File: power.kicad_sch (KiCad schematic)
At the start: 1 part, among them U40 RP2040

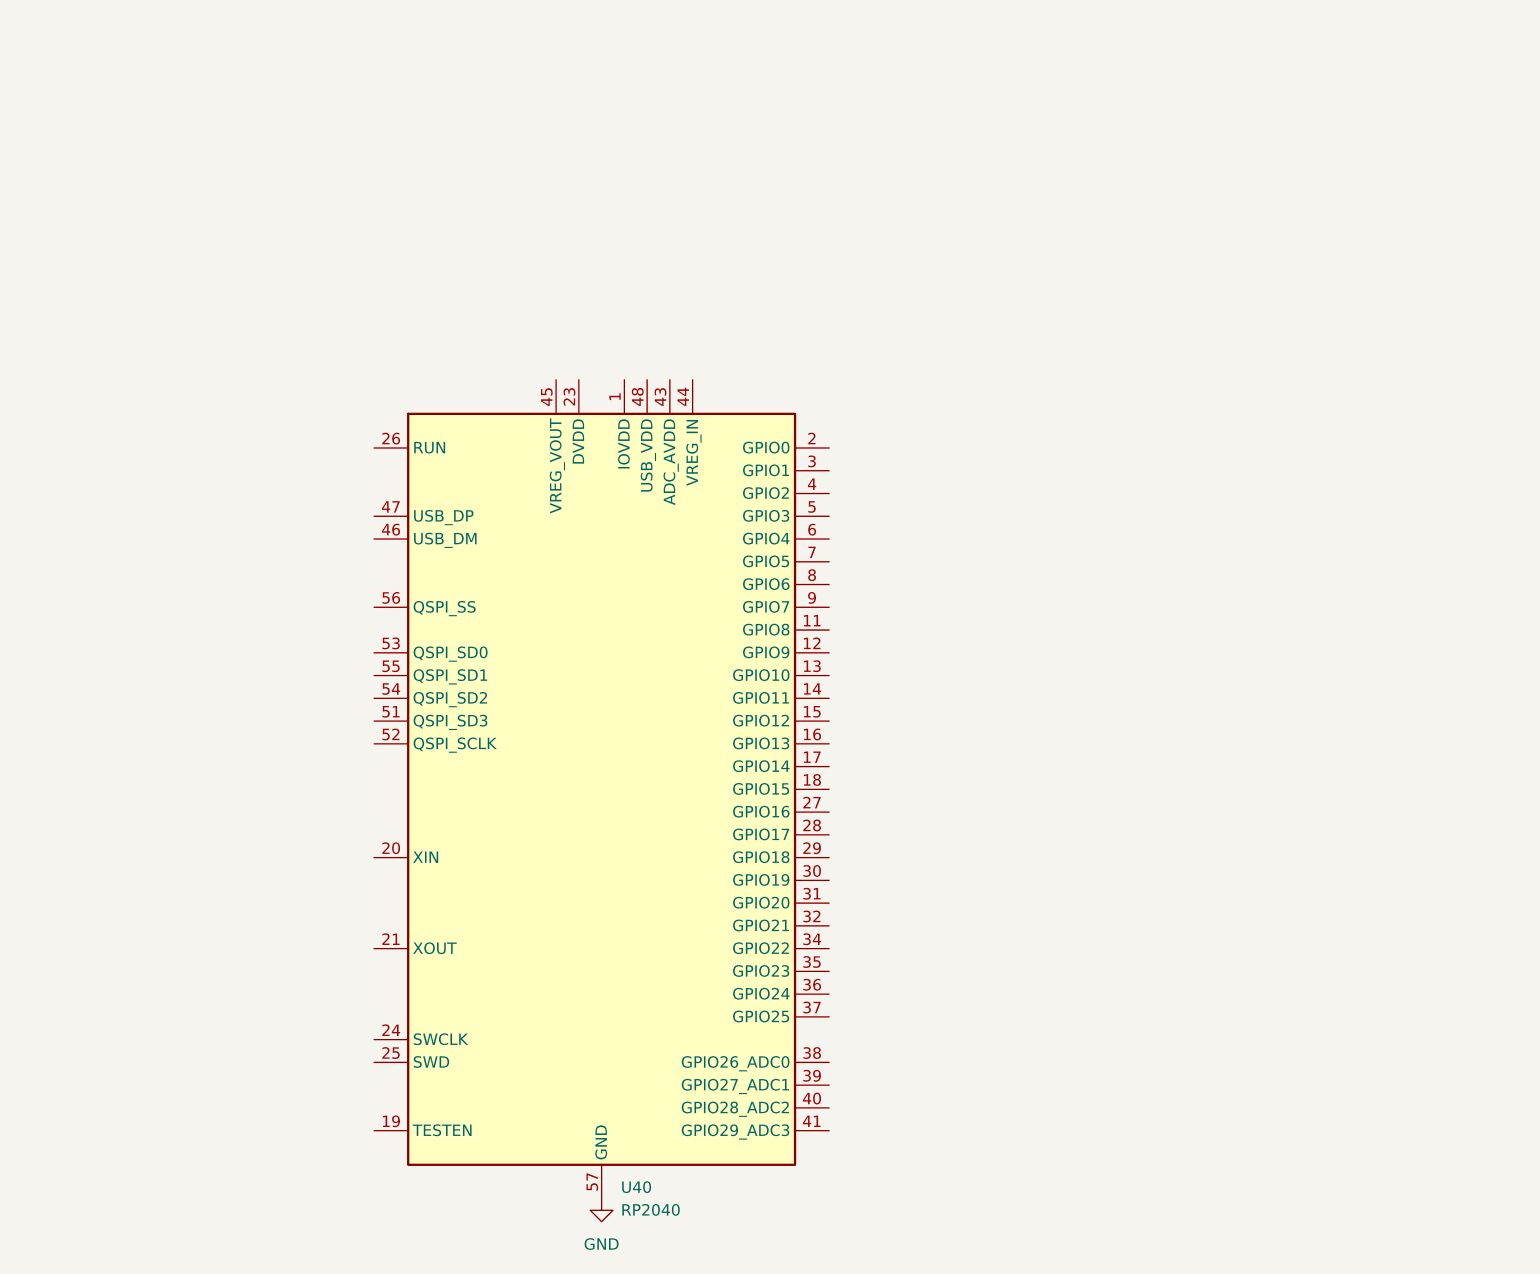
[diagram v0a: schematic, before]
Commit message: Before 10K resistors change
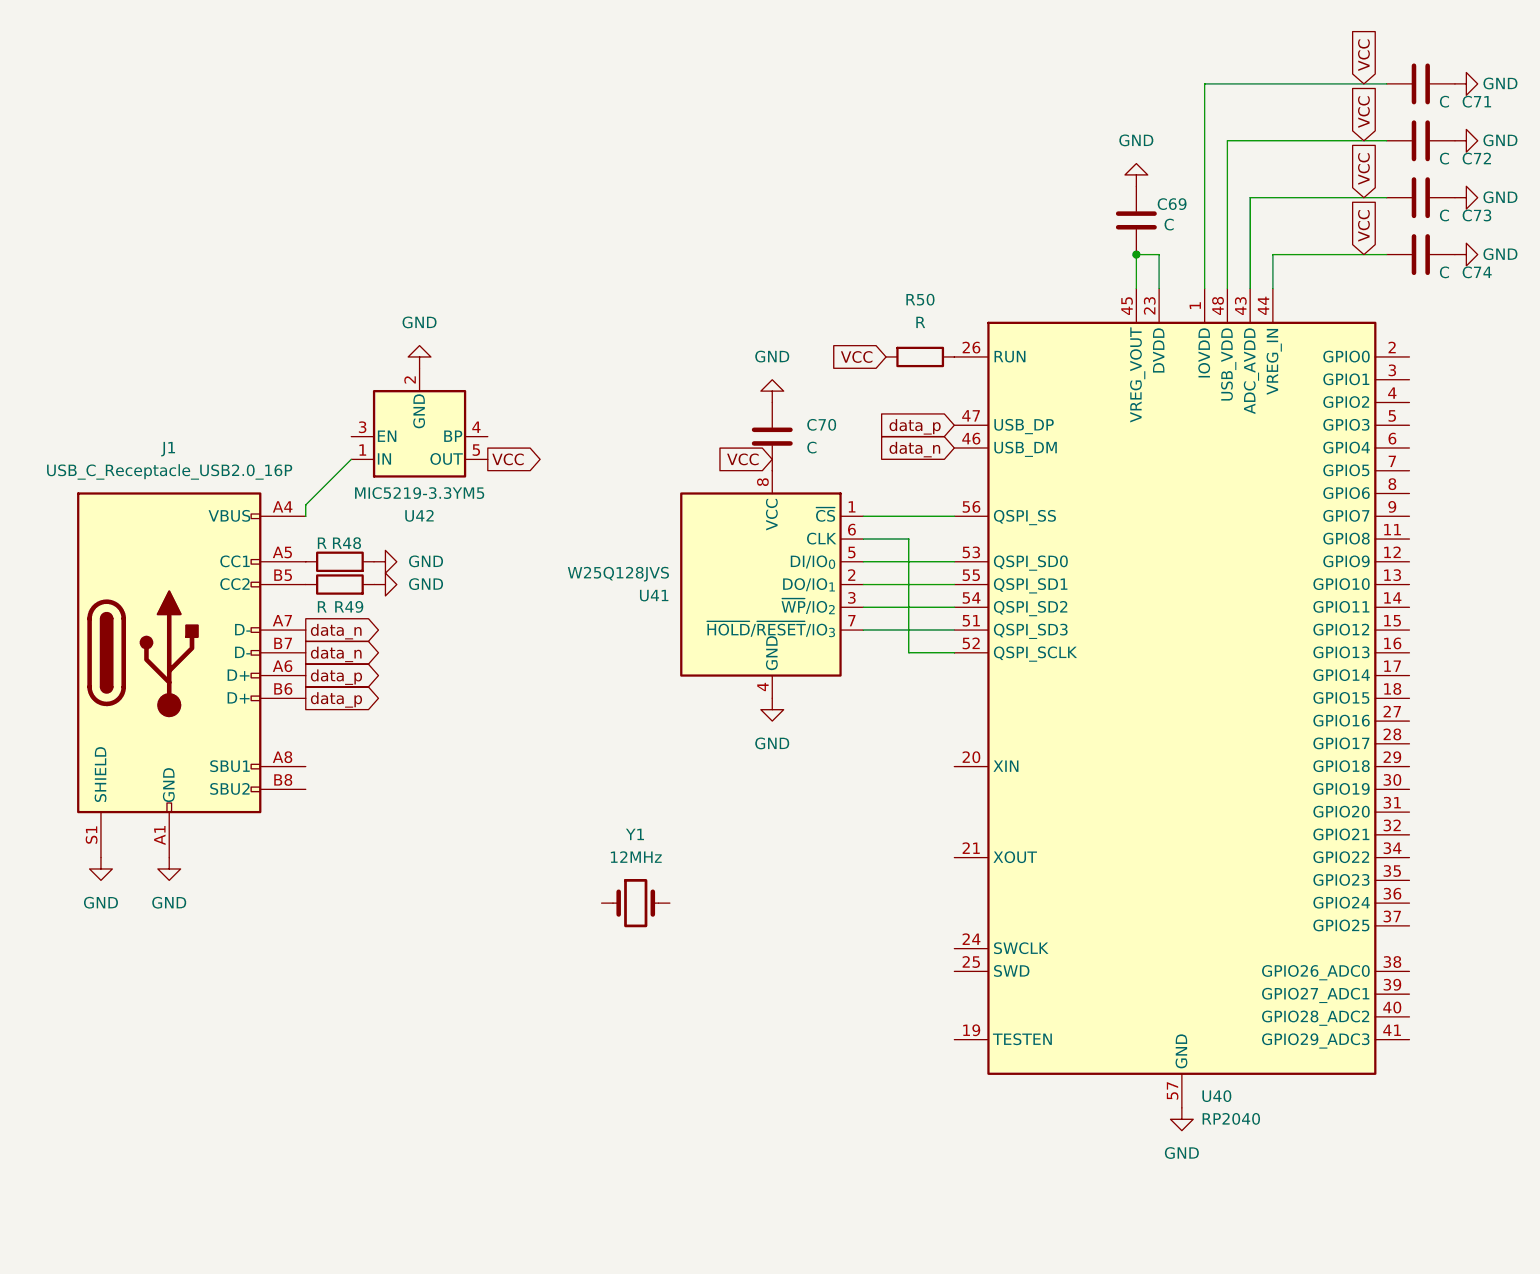
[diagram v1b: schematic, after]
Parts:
- added C69, C70, C71, C72, C73, C74: C, symbol Device:C
- added J1: USB_C_Receptacle_USB2.0_16P, symbol Connector:USB_C_Receptacle_USB2.0_16P
- added R48, R49, R50: R, symbol Device:R
- added U41: W25Q128JVS, Package_SO:SOIC-8_5.3x5.3mm_P1.27mm, symbol Memory_Flash:W25Q128JVS
- added U42: MIC5219-3.3YM5, Package_TO_SOT_SMD:SOT-23-5, symbol Regulator_Linear:MIC5219-3.3YM5
- added Y1: 12MHz, symbol Device:Crystal
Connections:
- net GND: now also C69.1, C70.1, C71.1, C72.1, C73.1, C74.1, J1.A1 (GND), J1.A12 (GND), J1.B1 (GND), J1.B12 (GND), J1.S1 (SHIELD), R48.2, R49.2, U41.4 (GND), U42.2 (GND)
- net VCC: now reaches U40.1 (IOVDD), U40.10 (IOVDD), U40.22 (IOVDD), U40.33 (IOVDD), U40.42 (IOVDD), U40.49 (IOVDD)
- net VCC: now also U40.43 (ADC_AVDD), U40.44 (VREG_IN), U40.48 (USB_VDD), C71.2, C72.2, C73.2, C74.2, R50.2, U42.5 (OUT)
- net at U40.23 (DVDD), U40.50 (DVDD): now also U40.45 (VREG_VOUT), C69.2
- net at U40.26 (RUN): now also R50.1
- net data_n: now reaches U40.46 (USB_DM)
- net data_n: now also J1.A7 (D-), J1.B7 (D-)
- net data_p: now reaches U40.47 (USB_DP)
- net data_p: now also J1.A6 (D+), J1.B6 (D+)
- net at U40.51 (QSPI_SD3): now also U41.7 (~{HOLD}/~{RESET}/IO_{3})
- net at U40.52 (QSPI_SCLK): now also U41.6 (CLK)
- net at U40.53 (QSPI_SD0): now also U41.5 (DI/IO_{0})
- net at U40.54 (QSPI_SD2): now also U41.3 (~{WP}/IO_{2})
- net at U40.55 (QSPI_SD1): now also U41.2 (DO/IO_{1})
- net at U40.56 (QSPI_SS): now also U41.1 (~{CS})
- new net: C70.2, U41.8 (VCC)
- new net: J1.A5 (CC1), R48.1
- new net: J1.A4 (VBUS), J1.A9 (VBUS), J1.B4 (VBUS), J1.B9 (VBUS), U42.1 (IN)
- new net: J1.B5 (CC2), R49.1
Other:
- moved on the sheet: U40
